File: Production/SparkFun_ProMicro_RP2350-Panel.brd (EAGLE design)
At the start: 92.7 x 87.1 mm, 732 parts, among them J1 QWIIC_RIGHT_ANGLE, J12 USB Female Type C Connector, J13 QWIIC_RIGHT_ANGLE, J16 USB Female Type C Connector, J17 QWIIC_RIGHT_ANGLE, J2 QWIIC_RIGHT_ANGLE, J20 USB Female Type C Connector, J21 QWIIC_RIGHT_ANGLE, J24 USB Female Type C Connector, J5 USB Female Type C Connector, J8 USB Female Type C Connector, J9 QWIIC_RIGHT_ANGLE, U1 RT9080-33GJ5, U10 APS6404L-3SQR-ZR, U11 RT9080-33GJ5, U12 W25QXX128MBIT, U13 WS2812_2020, U14 RP2350A, U15 APS6404L-3SQR-ZR, U16 RT9080-33GJ5, U17 W25QXX128MBIT, U18 WS2812_2020, U19 RP2350A, U2 RP2350A, U20 APS6404L-3SQR-ZR, U21 RT9080-33GJ5, U22 W25QXX128MBIT, U23 WS2812_2020, U24 RP2350A, U25 APS6404L-3SQR-ZR, U26 RT9080-33GJ5, U27 W25QXX128MBIT, U28 WS2812_2020, U29 RP2350A, U3 WS2812_2020, U30 APS6404L-3SQR-ZR, U4 W25QXX128MBIT, U5 APS6404L-3SQR-ZR, U6 RT9080-33GJ5, U7 W25QXX128MBIT, U8 WS2812_2020, U9 RP2350A, Y1 12MHz, Y2 12MHz, Y3 12MHz, Y4 12MHz, Y5 12MHz, Y6 12MHz

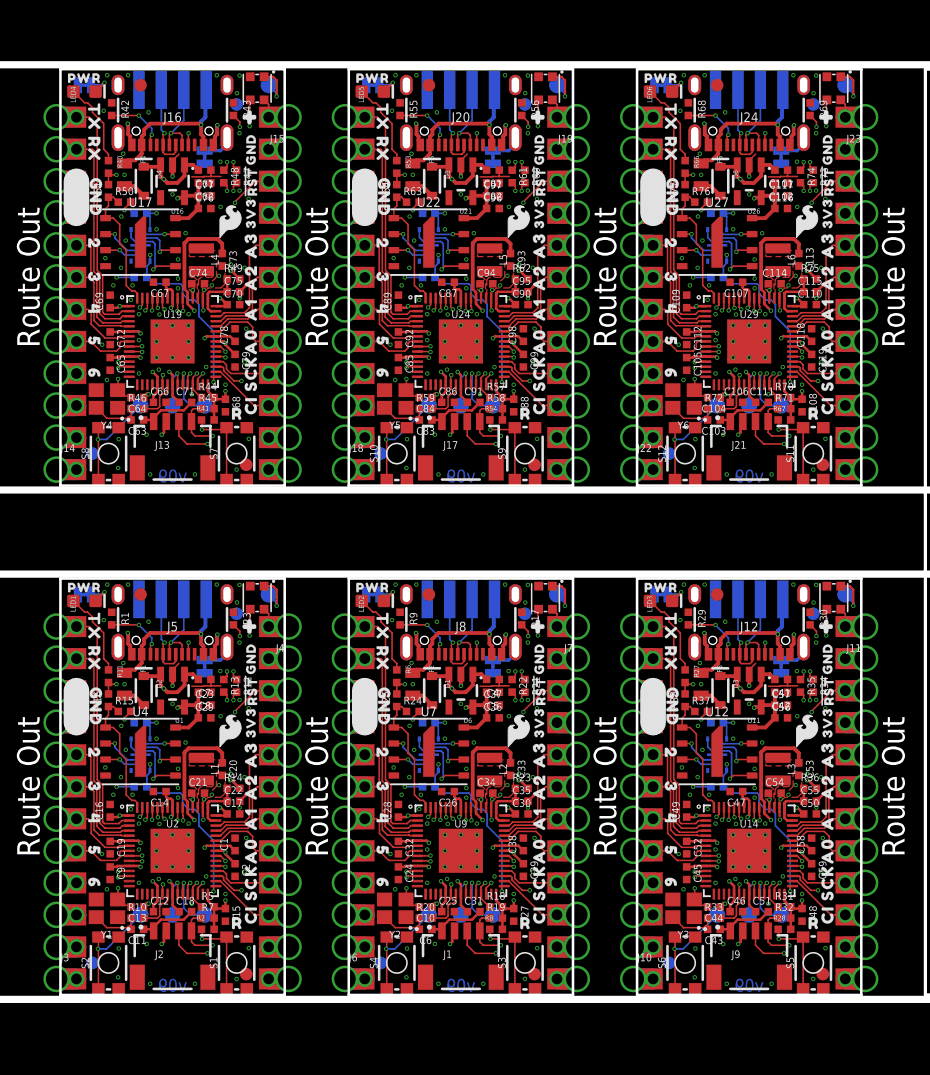
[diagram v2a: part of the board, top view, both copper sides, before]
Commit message: Add v02 panel files
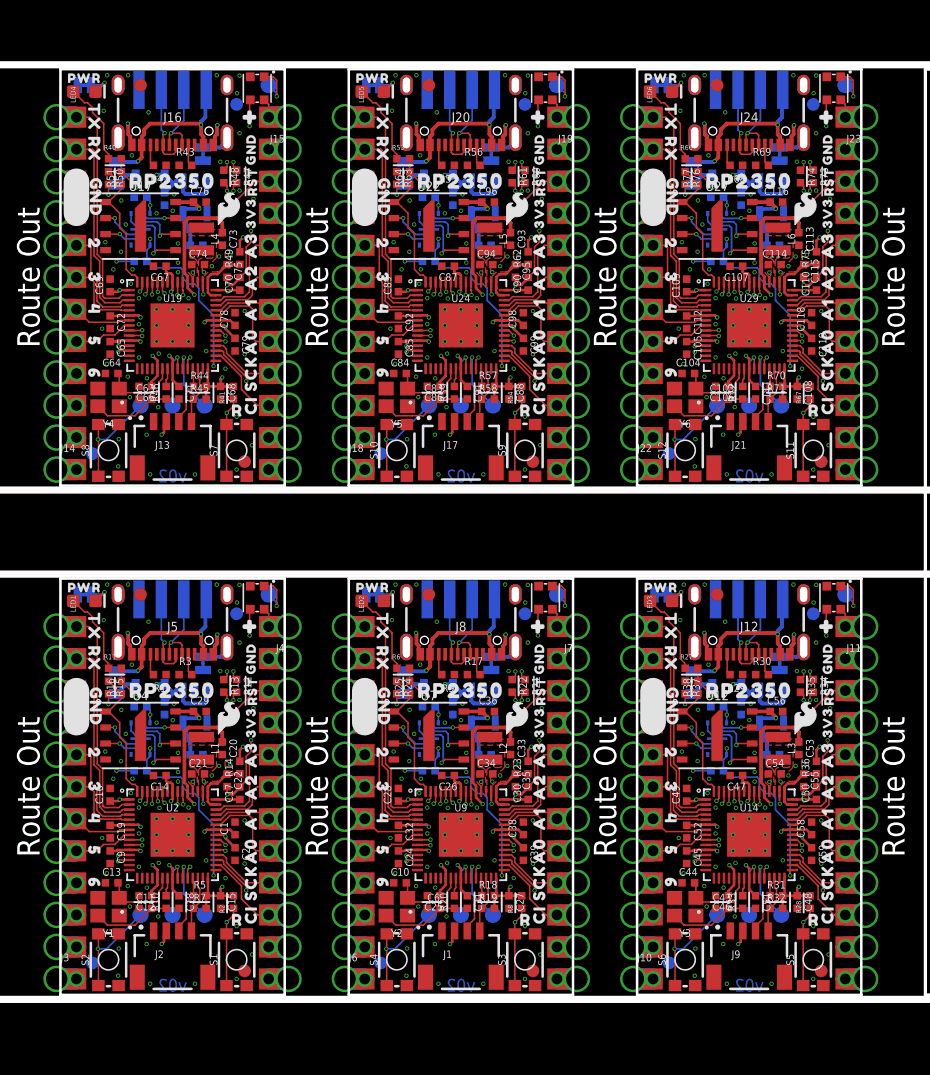
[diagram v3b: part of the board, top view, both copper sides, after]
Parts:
- added U$349: (no value), output:B0
- added U$350: (no value), output:#SHLD#0
- added U$351: (no value), output:#P#0
- added U$352: (no value), output:BOOT0
- added U$353: (no value), output:RST0
- added U$354: (no value), output:RP23500
- U$100: device output:210 -> output:V3
- U$101: device output:#RST#0 -> output:210
- U$102: device output:3V3_0 -> output:#RST#0
- U$103: device output:GND2 -> output:3V3_0
- U$104: device output:RAW0 -> output:GND2
- U$105: device output:R0 -> output:RAW0
- U$106: device output:#0 -> output:R0
- U$107: device output:PRO_MICRO0 -> output:#0
- U$108: device output:C0 -> output:PRO_MICRO0
- U$109: device output:D1 -> output:C0
- U$110: device output:DO0 -> output:D1
- U$111: device output:RP23500 -> output:DO0
- U$112: device output:B0 -> output:RP23500
- U$113: device output:#SHLD#0 -> output:B0
- U$114: device output:#P#0 -> output:#SHLD#0
- U$115: device output:BOOT0 -> output:#P#0
- U$116: device output:RST0 -> output:BOOT0
- U$117: value OSHW-LOGOMINI -> (none); device SparkFun-Aesthetics:OSHW-LOGO-MINI -> output:RST0
- U$118: device output:A00 -> output:RP23500
- U$119: value (none) -> OSHW-LOGOMINI; device output:A10 -> SparkFun-Aesthetics:OSHW-LOGO-MINI
- U$120, U$144: device output:A21 -> output:A00
- U$121, U$145: device output:A32 -> output:A10
- U$122: device output:CI4 -> output:A21
- U$123: device output:CO5 -> output:A32
- U$124, U$83: device output:SCK3 -> output:CI4
- U$125: device output:20 -> output:CO5
- U$126: device output:31 -> output:SCK3
- U$127, U$151: device output:42 -> output:20
- U$128, U$152: device output:53 -> output:31
- U$129, U$153: device output:64 -> output:42
- U$130: device output:#RST#1 -> output:53
- U$131: device output:3V30 -> output:64
- U$132: device output:PWR0 -> output:#RST#1
- U$133: device output:GND2 -> output:3V30
- U$134: device output:RX1 -> output:PWR0
- U$135: device output:TX0 -> output:GND2
- U$136: device output:GND_0 -> output:RX1
- U$137: device output:70 -> output:TX0
- U$138: device output:81 -> output:GND_0
- U$139: device output:92 -> output:70
- U$140: device output:CI4 -> output:81
- U$141: device output:SCK3 -> output:92
- U$142: device output:A00 -> output:CI4
- U$143: device output:A10 -> output:SCK3
- U$146: device output:TX0 -> output:A21
- U$147: device output:RX1 -> output:A32
- U$148: device output:GND2 -> output:TX0
- U$149: device output:20 -> output:RX1
- U$150: device output:31 -> output:GND2
- U$154: device output:D#1 -> output:53
- U$155: device output:D#2 -> output:64
- U$156: device output:G0 -> output:D#1
- U$157: device output:V3 -> output:D#2
- U$158: device output:210 -> output:G0
- U$159: device output:#RST#0 -> output:V3
- U$160: device output:3V3_0 -> output:210
- U$161: device output:GND2 -> output:#RST#0
- U$162: device output:RAW0 -> output:3V3_0
- U$163: device output:R0 -> output:GND2
- U$164: device output:#0 -> output:RAW0
- U$165: device output:PRO_MICRO0 -> output:R0
- U$166: device output:C0 -> output:#0
- U$167: device output:D1 -> output:PRO_MICRO0
- U$168: device output:DO0 -> output:C0
- U$169: device output:RP23500 -> output:D1
- U$170: device output:B0 -> output:DO0
- U$171: device output:#SHLD#0 -> output:RP23500
- U$172: device output:#P#0 -> output:B0
- U$173: device output:BOOT0 -> output:#SHLD#0
- U$174: device output:RST0 -> output:#P#0
- U$175: value OSHW-LOGOMINI -> (none); device SparkFun-Aesthetics:OSHW-LOGO-MINI -> output:BOOT0
- U$176: device output:A00 -> output:RST0
- U$177: device output:A10 -> output:RP23500
- U$178: value (none) -> OSHW-LOGOMINI; device output:A21 -> SparkFun-Aesthetics:OSHW-LOGO-MINI
- U$179, U$203: device output:A32 -> output:A00
- U$180: device output:CI4 -> output:A10
- U$181: device output:CO5 -> output:A21
- U$182: device output:SCK3 -> output:A32
- U$183: device output:20 -> output:CI4
- U$184: device output:31 -> output:CO5
- U$185: device output:42 -> output:SCK3
- U$186, U$210: device output:53 -> output:20
- U$187, U$211: device output:64 -> output:31
- U$188: device output:#RST#1 -> output:42
- U$189: device output:3V30 -> output:53
- U$190: device output:PWR0 -> output:64
- U$191: device output:GND2 -> output:#RST#1
- U$192: device output:RX1 -> output:3V30
- U$193: device output:TX0 -> output:PWR0
- U$194: device output:GND_0 -> output:GND2
- U$195: device output:70 -> output:RX1
- U$196: device output:81 -> output:TX0
- U$197: device output:92 -> output:GND_0
- U$198: device output:CI4 -> output:70
- U$199: device output:SCK3 -> output:81
- U$200: device output:A00 -> output:92
- U$201: device output:A10 -> output:CI4
- U$202: device output:A21 -> output:SCK3
- U$204: device output:TX0 -> output:A10
- U$205: device output:RX1 -> output:A21
- U$206: device output:GND2 -> output:A32
- U$207: device output:20 -> output:TX0
- U$208: device output:31 -> output:RX1
- U$209: device output:42 -> output:GND2
- U$212: device output:D#1 -> output:42
- U$213: device output:D#2 -> output:53
- U$214: device output:G0 -> output:64
- U$215: device output:V3 -> output:D#1
- U$216: device output:210 -> output:D#2
- U$217: device output:#RST#0 -> output:G0
- U$218: device output:3V3_0 -> output:V3
- U$219: device output:GND2 -> output:210
- U$220: device output:RAW0 -> output:#RST#0
- U$221: device output:R0 -> output:3V3_0
- U$222: device output:#0 -> output:GND2
- U$223: device output:PRO_MICRO0 -> output:RAW0
- U$224: device output:C0 -> output:R0
- U$225: device output:D1 -> output:#0
- U$226: device output:DO0 -> output:PRO_MICRO0
- U$227: device output:RP23500 -> output:C0
- U$228: device output:B0 -> output:D1
- U$229: device output:#SHLD#0 -> output:DO0
- U$230: device output:#P#0 -> output:RP23500
- U$231: device output:BOOT0 -> output:B0
- U$232: device output:RST0 -> output:#SHLD#0
- U$233: value OSHW-LOGOMINI -> (none); device SparkFun-Aesthetics:OSHW-LOGO-MINI -> output:#P#0
- U$234: device output:A00 -> output:BOOT0
- U$235: device output:A10 -> output:RST0
- U$236: device output:A21 -> output:RP23500
- U$237: value (none) -> OSHW-LOGOMINI; device output:A32 -> SparkFun-Aesthetics:OSHW-LOGO-MINI
- U$238: device output:CI4 -> output:A00
- U$239: device output:CO5 -> output:A10
- U$240: device output:SCK3 -> output:A21
- U$241, U$265: device output:20 -> output:A32
- U$242: device output:31 -> output:CI4
- U$243: device output:42 -> output:CO5
- U$244: device output:53 -> output:SCK3
- U$245, U$269: device output:64 -> output:20
- U$246: device output:#RST#1 -> output:31
- U$247: device output:3V30 -> output:42
- U$248: device output:PWR0 -> output:53
- U$249: device output:GND2 -> output:64
- U$250: device output:RX1 -> output:#RST#1
- U$251: device output:TX0 -> output:3V30
- U$252: device output:GND_0 -> output:PWR0
- U$253: device output:70 -> output:GND2
- U$254: device output:81 -> output:RX1
- U$255: device output:92 -> output:TX0
- U$256: device output:CI4 -> output:GND_0
- U$257: device output:SCK3 -> output:70
- U$258: device output:A00 -> output:81
- U$259: device output:A10 -> output:92
- U$260: device output:A21 -> output:CI4
- U$261: device output:A32 -> output:SCK3
- U$262: device output:TX0 -> output:A00
- U$263: device output:RX1 -> output:A10
- U$264: device output:GND2 -> output:A21
- U$266: device output:31 -> output:TX0
- U$267: device output:42 -> output:RX1
- U$268: device output:53 -> output:GND2
- U$270: device output:D#1 -> output:31
- U$271: device output:D#2 -> output:42
- U$272: device output:G0 -> output:53
- U$273: device output:V3 -> output:64
- U$274: device output:210 -> output:D#1
- U$275: device output:#RST#0 -> output:D#2
- U$276: device output:3V3_0 -> output:G0
- U$277: device output:GND2 -> output:V3
- U$278: device output:RAW0 -> output:210
- U$279: device output:R0 -> output:#RST#0
- U$280: device output:#0 -> output:3V3_0
- U$281: device output:PRO_MICRO0 -> output:GND2
- U$282: device output:C0 -> output:RAW0
- U$283: device output:D1 -> output:R0
- U$284: device output:DO0 -> output:#0
- U$285: device output:RP23500 -> output:PRO_MICRO0
- U$286: device output:B0 -> output:C0
- U$287: device output:#SHLD#0 -> output:D1
- U$288: device output:#P#0 -> output:DO0
- U$289: device output:BOOT0 -> output:RP23500
- U$290: device output:RST0 -> output:B0
- U$291: value OSHW-LOGOMINI -> (none); device SparkFun-Aesthetics:OSHW-LOGO-MINI -> output:#SHLD#0
- U$292: device output:A00 -> output:#P#0
- U$293: device output:A10 -> output:BOOT0
- U$294: device output:A21 -> output:RST0
- U$295: device output:A32 -> output:RP23500
- U$296: value (none) -> OSHW-LOGOMINI; device output:CI4 -> SparkFun-Aesthetics:OSHW-LOGO-MINI
- U$297: device output:CO5 -> output:A00
- U$298: device output:SCK3 -> output:A10
- U$299, U$323: device output:20 -> output:A21
- U$300, U$324: device output:31 -> output:A32
- U$301: device output:42 -> output:CI4
- U$302: device output:53 -> output:CO5
- U$303: device output:64 -> output:SCK3
- U$304: device output:#RST#1 -> output:20
- U$305: device output:3V30 -> output:31
- U$306: device output:PWR0 -> output:42
- U$307: device output:GND2 -> output:53
- U$308: device output:RX1 -> output:64
- U$309: device output:TX0 -> output:#RST#1
- U$310: device output:GND_0 -> output:3V30
- U$311: device output:70 -> output:PWR0
- U$312: device output:81 -> output:GND2
- U$313: device output:92 -> output:RX1
- U$314: device output:CI4 -> output:TX0
- U$315: device output:SCK3 -> output:GND_0
- U$316: device output:A00 -> output:70
- U$317: device output:A10 -> output:81
- U$318: device output:A21 -> output:92
- U$319: device output:A32 -> output:CI4
- U$320: device output:TX0 -> output:SCK3
- U$321: device output:RX1 -> output:A00
- U$322: device output:GND2 -> output:A10
- U$325: device output:42 -> output:TX0
- U$326: device output:53 -> output:RX1
- U$327: device output:64 -> output:GND2
- U$328: device output:D#1 -> output:20
- U$329: device output:D#2 -> output:31
- U$330: device output:G0 -> output:42
- U$331: device output:V3 -> output:53
- U$332: device output:210 -> output:64
- U$333: device output:#RST#0 -> output:D#1
- U$334: device output:3V3_0 -> output:D#2
- U$335: device output:GND2 -> output:G0
- U$336: device output:RAW0 -> output:V3
- U$337: device output:R0 -> output:210
- U$338: device output:#0 -> output:#RST#0
- U$339: device output:PRO_MICRO0 -> output:3V3_0
- U$340: device output:C0 -> output:GND2
- U$341: device output:D1 -> output:RAW0
- U$342: device output:DO0 -> output:R0
- U$343: device output:RP23500 -> output:#0
- U$344: device output:B0 -> output:PRO_MICRO0
- U$345: device output:#SHLD#0 -> output:C0
- U$346: device output:#P#0 -> output:D1
- U$347: device output:BOOT0 -> output:DO0
- U$348: device output:RST0 -> output:RP23500
- U$45: value OSHW-LOGOMINI -> (none); device SparkFun-Aesthetics:OSHW-LOGO-MINI -> output:RP23500
- U$46: value (none) -> OSHW-LOGOMINI; device output:A00 -> SparkFun-Aesthetics:OSHW-LOGO-MINI
- U$47, U$85: device output:A10 -> output:A00
- U$48, U$86: device output:A21 -> output:A10
- U$49, U$87: device output:A32 -> output:A21
- U$50: device output:CI4 -> output:A32
- U$51: device output:CO5 -> output:CI4
- U$52: device output:SCK3 -> output:CO5
- U$58: device output:20 -> output:SCK3
- U$59, U$92: device output:31 -> output:20
- U$60, U$93: device output:42 -> output:31
- U$61, U$94: device output:53 -> output:42
- U$62, U$95: device output:64 -> output:53
- U$63: device output:#RST#1 -> output:64
- U$65: device output:3V30 -> output:#RST#1
- U$70: device output:PWR0 -> output:3V30
- U$71: device output:GND2 -> output:PWR0
- U$72: device output:RX1 -> output:GND2
- U$77: device output:TX0 -> output:RX1
- U$78: device output:GND_0 -> output:TX0
- U$79: device output:70 -> output:GND_0
- U$80: device output:81 -> output:70
- U$81: device output:92 -> output:81
- U$82: device output:CI4 -> output:92
- U$84: device output:A00 -> output:SCK3
- U$88: device output:TX0 -> output:A32
- U$89: device output:RX1 -> output:TX0
- U$90: device output:GND2 -> output:RX1
- U$91: device output:20 -> output:GND2
- U$96: device output:D#1 -> output:64
- U$97: device output:D#2 -> output:D#1
- U$98: device output:G0 -> output:D#2
- U$99: device output:V3 -> output:G0
- moved U$175 66.2 mm to (51.3, 2.54), turned to 0 degrees
- moved U$176 65.1 mm to (57.7, 2.54), flipped to the bottom, turned to 0 degrees
- moved U$177 49.7 mm to (54.6, 24.1), turned to 0 degrees
- moved U$292 39.5 mm to (26.2, 70.7), flipped to the bottom, turned to 0 degrees
- moved U$293 34.3 mm to (28.4, 42.9), flipped to the bottom, turned to 0 degrees
- moved U$234 33.6 mm to (5.59, 42.9), flipped to the bottom, turned to 0 degrees
- moved U$233 32.3 mm to (3.30, 70.7), turned to 0 degrees
- moved U$118 31.7 mm to (31.8, 24.1), turned to 0 degrees
- moved U$347 30.6 mm to (60.7, 72.0), turned to 270 degrees
- moved U$236 30.1 mm to (8.89, 64.5), turned to 0 degrees
- moved U$294 29.5 mm to (34.8, 42.9), flipped to the bottom, turned to 0 degrees
- moved U$295 29.5 mm to (31.8, 64.5), turned to 0 degrees
- moved U$174 29.1 mm to (49.0, 30.4)
- moved U$158 29.0 mm to (51.9, 29.1), turned to 270 degrees
- moved U$235 28.4 mm to (11.9, 42.9), flipped to the bottom, turned to 0 degrees
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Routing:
- net 16/SDA2: track 12.0 -> 4.69 mm, vias 2 -> 0
- net 16/SDA5: track 12.0 -> 4.69 mm, vias 2 -> 0
- net 16/SDA: track 12.0 -> 4.69 mm, vias 2 -> 0
- net 16/SDA3: track 12.0 -> 4.69 mm, vias 2 -> 0
- net 16/SDA1: track 12.0 -> 4.69 mm, vias 2 -> 0
- net 16/SDA4: track 12.0 -> 4.69 mm, vias 2 -> 0
- net 17/SCL5: track 10.7 -> 4.62 mm, vias 2 -> 0
- net 17/SCL2: track 10.7 -> 4.62 mm, vias 2 -> 0
- net 17/SCL3: track 10.7 -> 4.62 mm, vias 2 -> 0
- net 17/SCL: track 10.7 -> 4.62 mm, vias 2 -> 0
- net 17/SCL4: track 10.7 -> 4.62 mm, vias 2 -> 0
- net 17/SCL1: track 10.7 -> 4.62 mm, vias 2 -> 0
- net N$4: track 7.29 -> 1.72 mm, vias 2 -> 0
- net N$11: track 7.29 -> 1.72 mm, vias 2 -> 0
- net N$9: track 7.29 -> 1.72 mm, vias 2 -> 0
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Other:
- board text added: "v02"
- board text removed: "v09"
